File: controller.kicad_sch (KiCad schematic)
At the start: 13 parts, among them J2 UART, J3 SWD, SW4 RST, U10 STM32C031K6Tx

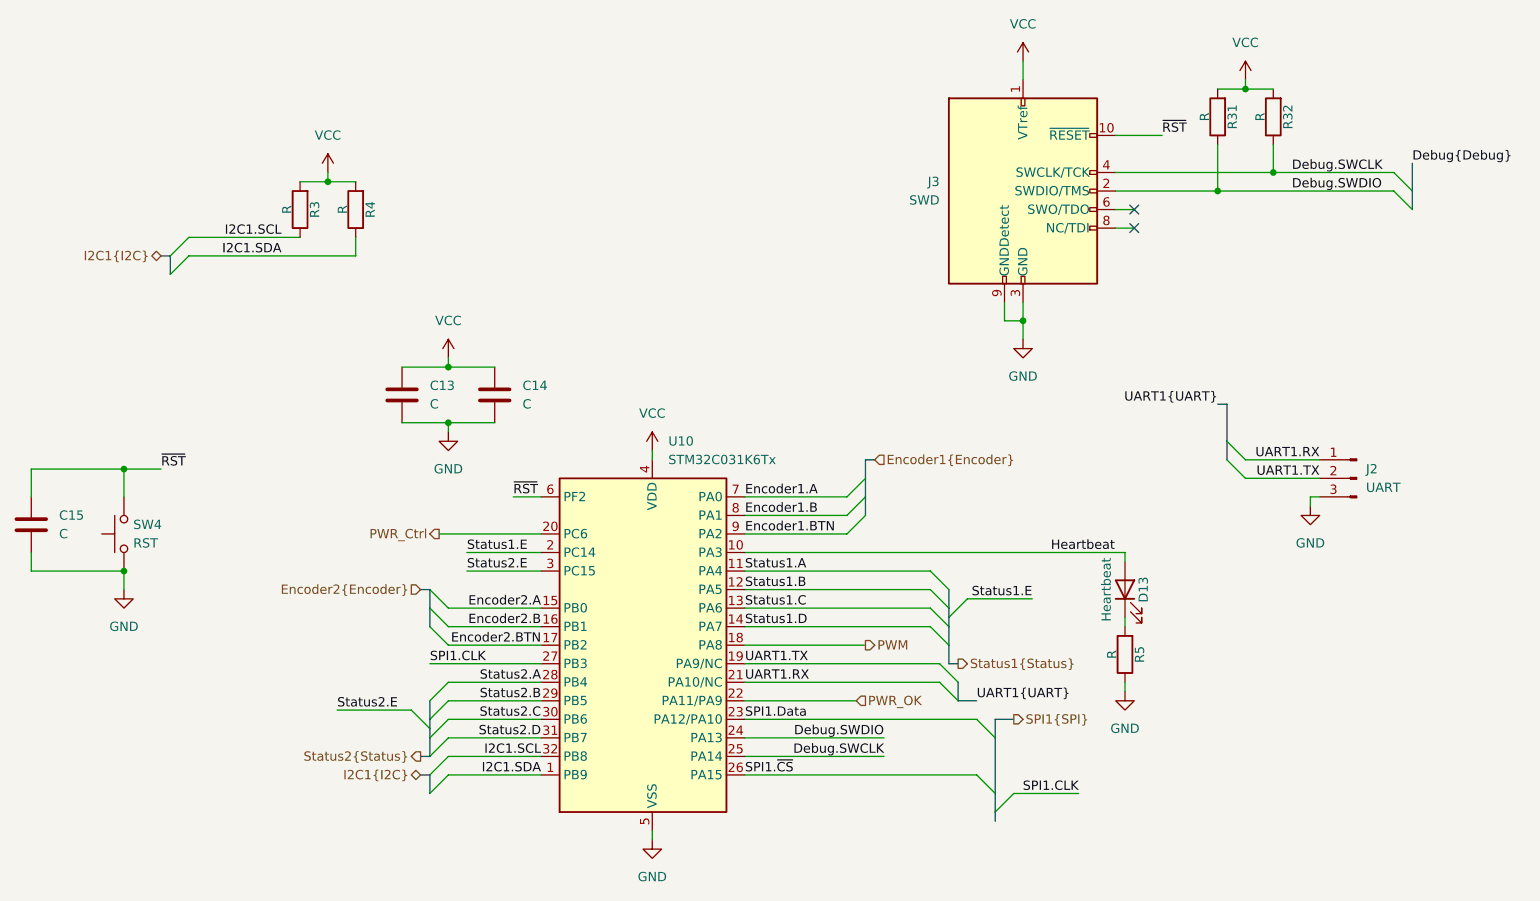
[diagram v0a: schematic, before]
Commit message: Initial layout
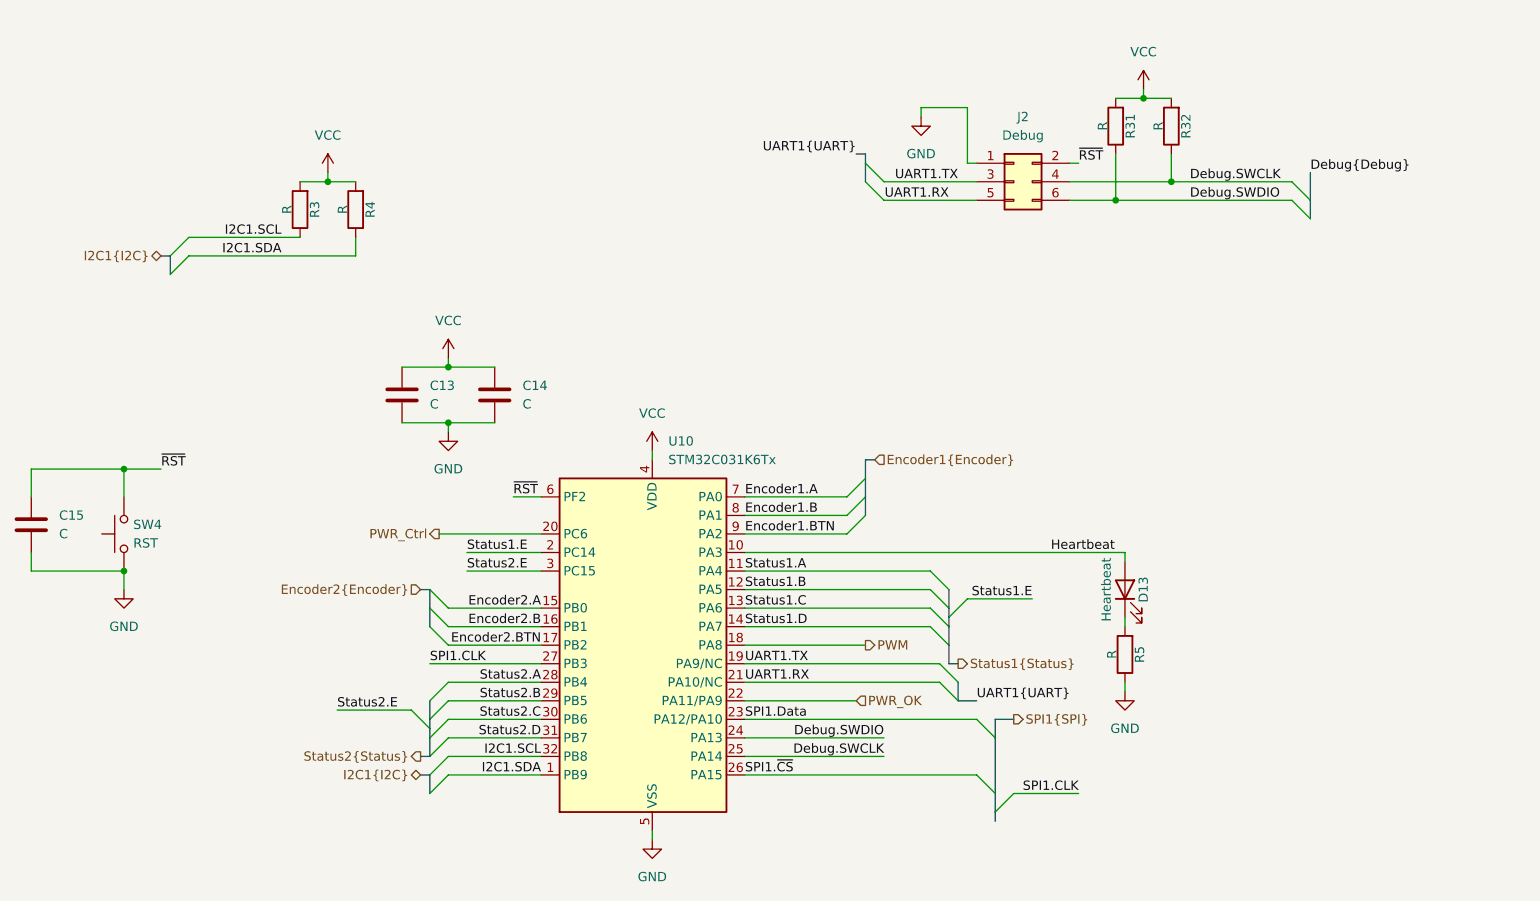
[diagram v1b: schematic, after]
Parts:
- removed J2: UART, Connector_PinHeader_2.54mm:PinHeader_1x03_P2.54mm_Vertical_SMD_Pin1Left, symbol Connector:Conn_01x03_Pin
- removed J3: SWD, Connector_PinHeader_1.27mm:PinHeader_2x05_P1.27mm_Vertical_SMD, symbol Connector:Conn_ARM_JTAG_SWD_10
- added J2: Debug, Connector_PinHeader_2.54mm:PinHeader_2x03_P2.54mm_Vertical_SMD, symbol Connector_Generic:Conn_02x03_Odd_Even
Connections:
- net Debug.SWCLK: now also J2.4 (Pin_4)
- net Debug.SWDIO: now also J2.6 (Pin_6)
- net GND: now also J2.1 (Pin_1)
- net UART1.RX: now also J2.5 (Pin_5)
- net UART1.TX: now also J2.3 (Pin_3)
- net ~{RST}: now also J2.2 (Pin_2)
- no-connect marks 2 -> 0
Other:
- moved on the sheet: R31, R32
